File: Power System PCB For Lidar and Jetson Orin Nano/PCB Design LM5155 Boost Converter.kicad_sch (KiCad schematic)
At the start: 74 parts, among them J1 Conn_01x04_Pin, J2 B5B-XH-A, J5 BM06B-SRSS-TBLFSN, J6 B4B-XH-A, Q1 BSC035N04LS G, Q2 BSC035N04LS G, U1 LM5155_DSSR, U2 TPS552892RYQR

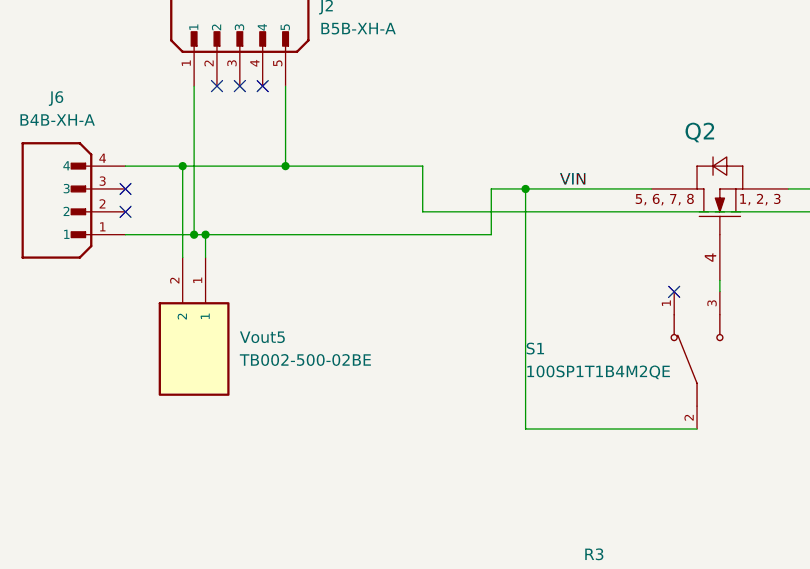
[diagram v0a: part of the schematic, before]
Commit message: Adjust some stuff
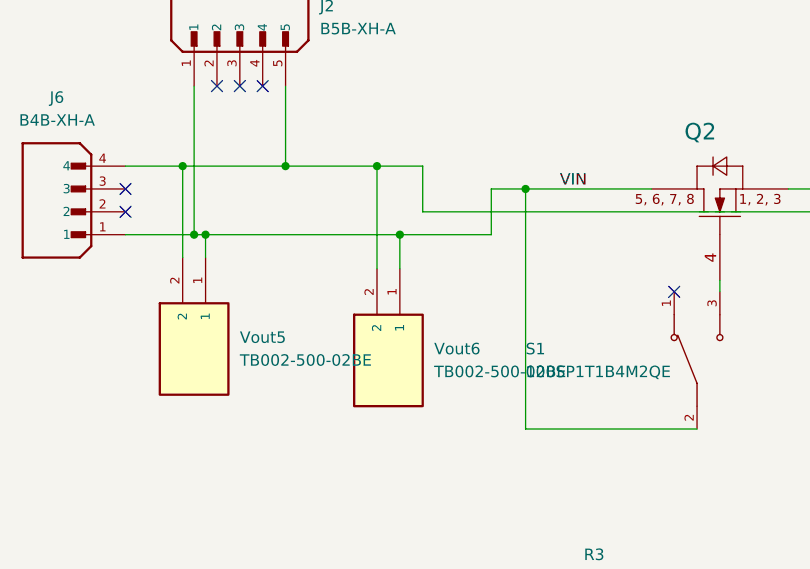
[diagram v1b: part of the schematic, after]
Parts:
- added Vout6: TB002-500-02BE, 282834-2:TE_282834-2, symbol TB002-500-02BE:TB002-500-02BE
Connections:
- net GNDPWR: now also Vout6.2
- net VIN: now also Vout6.1
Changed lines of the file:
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@@
 	)
 	(junction
+		(at 68.58 55.88)
+		(diameter 0)
+		(color 0 0 0 0)
+	)
+	(junction
 		(at 347.98 50.8)
 		(diameter 0)
@@
 	)
 	(junction
+		(at 66.04 48.26)
+		(diameter 0)
+		(color 0 0 0 0)
+	)
+	(junction
 		(at 292.1 69.85)
 		(diameter 0)
@@
 	(wire
 		(pts
-			(xy 46.99 55.88) (xy 78.74 55.88)
+			(xy 46.99 55.88) (xy 68.58 55.88)
 		)
 		(stroke
@@
 	(wire
 		(pts
-			(xy 71.12 48.26) (xy 55.88 48.26)
+			(xy 71.12 48.26) (xy 66.04 48.26)
 		)
 		(stroke
@@
 	(wire
 		(pts
+			(xy 66.04 48.26) (xy 66.04 59.69)
+		)
+		(stroke
+			(width 0)
+			(type default)
+		)
+	)
+	(wire
+		(pts
 			(xy 283.21 273.05) (xy 283.21 278.13)
 		)
@@
 	(wire
 		(pts
+			(xy 66.04 48.26) (xy 55.88 48.26)
+		)
+		(stroke
+			(width 0)
+			(type default)
+		)
+	)
+	(wire
+		(pts
 			(xy 275.59 215.9) (xy 275.59 218.44)
 		)
@@
 	(wire
 		(pts
+			(xy 68.58 55.88) (xy 78.74 55.88)
+		)
+		(stroke
+			(width 0)
+			(type default)
+		)
+	)
+	(wire
+		(pts
 			(xy 425.45 63.5) (xy 425.45 66.04)
 		)
@@
 	(wire
 		(pts
+			(xy 68.58 55.88) (xy 68.58 59.69)
+		)
+		(stroke
+			(width 0)
+			(type default)
+		)
+	)
+	(wire
+		(pts
 			(xy 464.82 66.675) (xy 464.82 63.5)
 		)
@@
 					(unit 1)
 				)
+			)
+		)
+	)
+	(symbol
+		(lib_id "TB002-500-02BE:TB002-500-02BE")
+		(at 66.04 69.85 270)
+		(unit 1)
+		(body_style 1)
+		(exclude_from_sim no)
+		(in_bom yes)
+		(on_board yes)
+		(in_pos_files yes)
+		(dnp no)
+		(fields_autoplaced yes)
+		(property "Reference" "Vout6"
+			(at 72.39 68.5799 90)
+			(show_name no)
+			(do_not_autoplace no)
+			(effects
+				(font
+					(size 1.27 1.27)
+				)
+				(justify left)
+			)
+		)
+		(property "Value" "TB002-500-02BE"
+			(at 72.39 71.1199 90)
+			(show_name no)
+			(do_not_autoplace no)
+			(effects
+				(font
+					(size 1.27 1.27)
+				)
+				(justify left)
+			)
+		)
+		(property "Footprint" "282834-2:TE_282834-2"
+			(at 66.04 69.85 0)
+			(hide yes)
+			(show_name no)
+			(do_not_autoplace no)
+			(effects
+				(font
+					(size 1.27 1.27)
+				)
+				(justify bottom)
+			)
+		)
+		(property "Datasheet" ""
+			(at 66.04 69.85 0)
+			(hide yes)
+			(show_name no)
+			(do_not_autoplace no)
+			(effects
+				(font
+					(size 1.27 1.27)
+				)
+			)
+		)
+		(property "Description" ""
+			(at 66.04 69.85 0)
+			(hide yes)
+			(show_name no)
+			(do_not_autoplace no)
+			(effects
+				(font
+					(size 1.27 1.27)
+				)
+			)
+		)
+		(property "STANDARD" "Manufacturer Recommendations"
+			(at 66.04 69.85 0)
+			(hide yes)
+			(show_name no)
+			(do_not_autoplace no)
+			(effects
+				(font
+					(size 1.27 1.27)
+				)
+				(justify bottom)
+			)
+		)
+		(property "MANUFACTURER" "CUI"
+			(at 66.04 69.85 0)
+			(hide yes)
+			(show_name no)
+			(do_not_autoplace no)
+			(effects
+				(font
+					(size 1.27 1.27)
+				)
+				(justify bottom)
+			)
+		)
+		(pin "1"
+		)
+		(pin "2"
+		)
+		(instances
+			(project "PCB Design LM5155 Boost Converter"
+				(path "/085c1d8f-d12d-46a1-b7b5-945f7ea1ec15"
+					(reference "Vout6")
+					(unit 1)
+				)
